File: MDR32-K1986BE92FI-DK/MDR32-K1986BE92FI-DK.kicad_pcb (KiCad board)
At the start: 2 copper layers, 69.6 x 21.4 mm, 56 parts, among them J1 Conn_PROBE, J2 PIN_A, J3 SYS_A, J4 USB_C_Receptacle_USB2.0_16P, J5 PIN_B, J6 SYS_B, Q1 AO3401A, SW1 IT-1181, SW2 SW_DIP_x02, SW3 IT-1181, U1 LM1117GS-3.3, Y1 SMD3225 P4 16MHz, Y2 32.768KHz ±20ppm 6pF

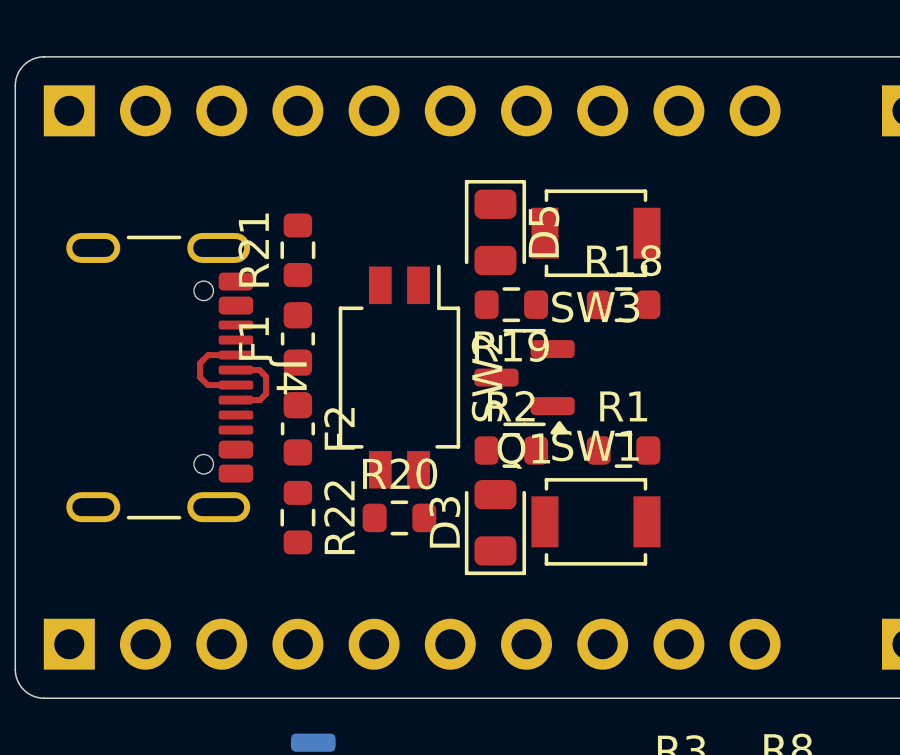
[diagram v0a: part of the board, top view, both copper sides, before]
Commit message: part position
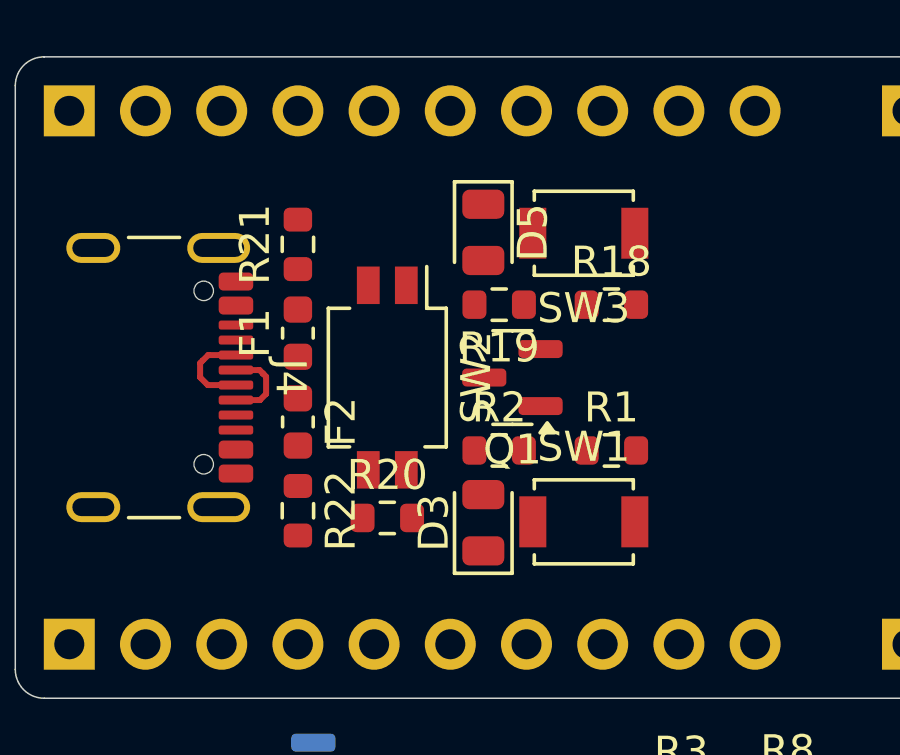
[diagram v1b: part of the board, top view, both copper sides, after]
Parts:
- moved D3 0.41 mm to (32.6, 32.6)
- moved D5 0.41 mm to (32.6, 22.9)
- moved Q1 0.41 mm to (33.6, 27.7)
- moved R1 0.41 mm to (36.9, 30.2)
- moved R18 0.41 mm to (36.9, 25.3)
- moved R19 0.41 mm to (33.2, 25.3)
- moved R2 0.41 mm to (33.2, 30.2)
- moved SW1 0.41 mm to (36.0, 32.5)
- moved SW3 0.41 mm to (36.0, 22.9)
- moved R20 0.40 mm to (29.4, 32.4)
- moved SW2 0.40 mm to (29.4, 27.7)
- moved F2 0.23 mm to (26.5, 29.2)
- moved R22 0.23 mm to (26.5, 32.2)
- moved R21 0.20 mm to (26.5, 23.3)
- moved F1 0.19 mm to (26.5, 26.2)
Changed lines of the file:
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@@
 	(footprint "LED_SMD:LED_0805_2012Metric"
 		(layer "F.Cu")
-		(at 33.045 22.89 -90)
+		(at 32.64 22.89 -90)
 		(descr "LED SMD 0805 (2012 Metric), square (rectangular) end terminal, IPC_7351 nominal, (Body size source: https://docs.google.com/spreadsheets/d/1BsfQQcO9C6DZCsRaXUlFlo91Tg2WpOkGARC1WS5S8t0/edit?usp=sharing), generated with kicad-footprint-generator")
 		(tags "LED")
@@
 	(footprint "Resistor_SMD:R_0603_1608Metric"
 		(layer "F.Cu")
-		(at 26.46 32.4 -90)
+		(at 26.46 32.17 -90)
 		(descr "Resistor SMD 0603 (1608 Metric), square (rectangular) end terminal, IPC_7351 nominal, (Body size source: IPC-SM-782 page 72, https://www.pcb-3d.com/wordpress/wp-content/uploads/ipc-sm-782a_amendment_1_and_2.pdf), generated with kicad-footprint-generator")
 		(tags "resistor")
@@
 	(footprint "Fuse:Fuse_0603_1608Metric"
 		(layer "F.Cu")
-		(at 26.46 26.4425 90)
+		(at 26.46 26.25 90)
 		(descr "Fuse SMD 0603 (1608 Metric), square (rectangular) end terminal, IPC_7351 nominal, (Body size source: http://www.tortai-tech.com/upload/download/2011102023233369053.pdf), generated with kicad-footprint-generator")
 		(tags "fuse")
@@
 	(footprint "Resistor_SMD:R_0603_1608Metric"
 		(layer "F.Cu")
-		(at 33.575 30.16)
+		(at 33.17 30.16)
 		(descr "Resistor SMD 0603 (1608 Metric), square (rectangular) end terminal, IPC_7351 nominal, (Body size source: IPC-SM-782 page 72, https://www.pcb-3d.com/wordpress/wp-content/uploads/ipc-sm-782a_amendment_1_and_2.pdf), generated with kicad-footprint-generator")
 		(tags "resistor")
@@
 	(footprint "Resistor_SMD:R_0603_1608Metric"
 		(layer "F.Cu")
-		(at 37.315 25.3)
+		(at 36.91 25.3)
 		(descr "Resistor SMD 0603 (1608 Metric), square (rectangular) end terminal, IPC_7351 nominal, (Body size source: IPC-SM-782 page 72, https://www.pcb-3d.com/wordpress/wp-content/uploads/ipc-sm-782a_amendment_1_and_2.pdf), generated with kicad-footprint-generator")
 		(tags "resistor")
@@
 	(footprint "Resistor_SMD:R_0603_1608Metric"
 		(layer "F.Cu")
-		(at 26.46 23.485 90)
+		(at 26.46 23.29 90)
 		(descr "Resistor SMD 0603 (1608 Metric), square (rectangular) end terminal, IPC_7351 nominal, (Body size source: IPC-SM-782 page 72, https://www.pcb-3d.com/wordpress/wp-content/uploads/ipc-sm-782a_amendment_1_and_2.pdf), generated with kicad-footprint-generator")
 		(tags "resistor")
@@
 	(footprint "Resistor_SMD:R_0603_1608Metric"
 		(layer "F.Cu")
-		(at 29.845 32.41)
+		(at 29.44 32.41)
 		(descr "Resistor SMD 0603 (1608 Metric), square (rectangular) end terminal, IPC_7351 nominal, (Body size source: IPC-SM-782 page 72, https://www.pcb-3d.com/wordpress/wp-content/uploads/ipc-sm-782a_amendment_1_and_2.pdf), generated with kicad-footprint-generator")
 		(tags "resistor")
@@
 	(footprint "Button_Switch_SMD:SW_SPST_B3U-1000P"
 		(layer "F.Cu")
-		(at 36.395 22.92 180)
+		(at 35.99 22.92 180)
 		(descr "Ultra-small-sized Tactile Switch with High Contact Reliability, Top-actuated Model, without Ground Terminal, without Boss")
 		(tags "Tactile Switch")
@@
 	(footprint "Button_Switch_SMD:SW_SPST_B3U-1000P"
 		(layer "F.Cu")
-		(at 36.395 32.54)
+		(at 35.99 32.54)
 		(descr "Ultra-small-sized Tactile Switch with High Contact Reliability, Top-actuated Model, without Ground Terminal, without Boss")
 		(tags "Tactile Switch")
@@
 	(footprint "Fuse:Fuse_0603_1608Metric"
 		(layer "F.Cu")
-		(at 26.46 29.44 -90)
+		(at 26.46 29.21 -90)
 		(descr "Fuse SMD 0603 (1608 Metric), square (rectangular) end terminal, IPC_7351 nominal, (Body size source: http://www.tortai-tech.com/upload/download/2011102023233369053.pdf), generated with kicad-footprint-generator")
 		(tags "fuse")
@@
 	(footprint "Resistor_SMD:R_0603_1608Metric"
 		(layer "F.Cu")
-		(at 37.315 30.16)
+		(at 36.91 30.16)
 		(descr "Resistor SMD 0603 (1608 Metric), square (rectangular) end terminal, IPC_7351 nominal, (Body size source: IPC-SM-782 page 72, https://www.pcb-3d.com/wordpress/wp-content/uploads/ipc-sm-782a_amendment_1_and_2.pdf), generated with kicad-footprint-generator")
 		(tags "resistor")
@@
 		(tags "capacitor")
 		(property "Reference" "C11"
-			(at 0 -1.43 360)
+			(at 0 -1.43 0)
 			(layer "F.SilkS")
 			(effects
@@
 		)
 		(property "Value" "0.1µF"
-			(at 0 1.43 360)
+			(at 0 1.43 0)
 			(layer "F.Fab")
 			(effects
@@
 		)
 		(fp_text user "${REFERENCE}"
-			(at 0 0 360)
+			(at 0 0 0)
 			(layer "F.Fab")
 			(effects
@@
 	(footprint "LED_SMD:LED_0805_2012Metric"
 		(layer "F.Cu")
-		(at 33.045 32.57 90)
+		(at 32.64 32.57 90)
 		(descr "LED SMD 0805 (2012 Metric), square (rectangular) end terminal, IPC_7351 nominal, (Body size source: https://docs.google.com/spreadsheets/d/1BsfQQcO9C6DZCsRaXUlFlo91Tg2WpOkGARC1WS5S8t0/edit?usp=sharing), generated with kicad-footprint-generator")
 		(tags "LED")
@@
 	(footprint "Package_TO_SOT_SMD:SOT-23"
 		(layer "F.Cu")
-		(at 34.015 27.73 180)
+		(at 33.61 27.73 180)
 		(descr "SOT, 3 Pin (JEDEC TO-236 Var AB https://www.jedec.org/document_search?search_api_views_fulltext=TO-236), generated with kicad-footprint-generator ipc_gullwing_generator.py")
 		(tags "SOT TO_SOT_SMD")
@@
 	(footprint "Button_Switch_SMD:SW_DIP_SPSTx02_Slide_Omron_A6H-2101_W6.15mm_P1.27mm"
 		(layer "F.Cu")
-		(at 29.845 27.73 -90)
+		(at 29.44 27.73 -90)
 		(descr "SMD 2x-dip-switch SPST Omron_A6H-2101, Slide, row spacing 6.15 mm (242 mils), body size  (see https://www.omron.com/ecb/products/pdf/en-a6h.pdf)")
 		(tags "SMD DIP Switch SPST Slide 6.15mm 242mil")
@@
 	(footprint "Resistor_SMD:R_0603_1608Metric"
 		(layer "F.Cu")
-		(at 33.575 25.3 180)
+		(at 33.17 25.3 180)
 		(descr "Resistor SMD 0603 (1608 Metric), square (rectangular) end terminal, IPC_7351 nominal, (Body size source: IPC-SM-782 page 72, https://www.pcb-3d.com/wordpress/wp-content/uploads/ipc-sm-782a_amendment_1_and_2.pdf), generated with kicad-footprint-generator")
 		(tags "resistor")
 		(property "Reference" "R19"
-			(at 0 -1.43 360)
+			(at 0 -1.43 0)
 			(layer "F.SilkS")
 			(effects
@@
 		)
 		(property "Value" "1k"
-			(at 0 1.43 360)
+			(at 0 1.43 0)
 			(layer "F.Fab")
 			(effects
@@
 		)
 		(fp_text user "${REFERENCE}"
-			(at 0 0 360)
+			(at 0 0 0)
 			(layer "F.Fab")
 			(effects
